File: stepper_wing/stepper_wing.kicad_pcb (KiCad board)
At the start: 2 copper layers, 47 x 49.5 mm, 39 parts, among them M1 Nylon, M2 Nylon, P1 24V, P2 GND, U1 MCP44X1, U2 MCP23017, U3 DRV8825, U4 DRV8825, U5 DRV8825, U6 DRV8825

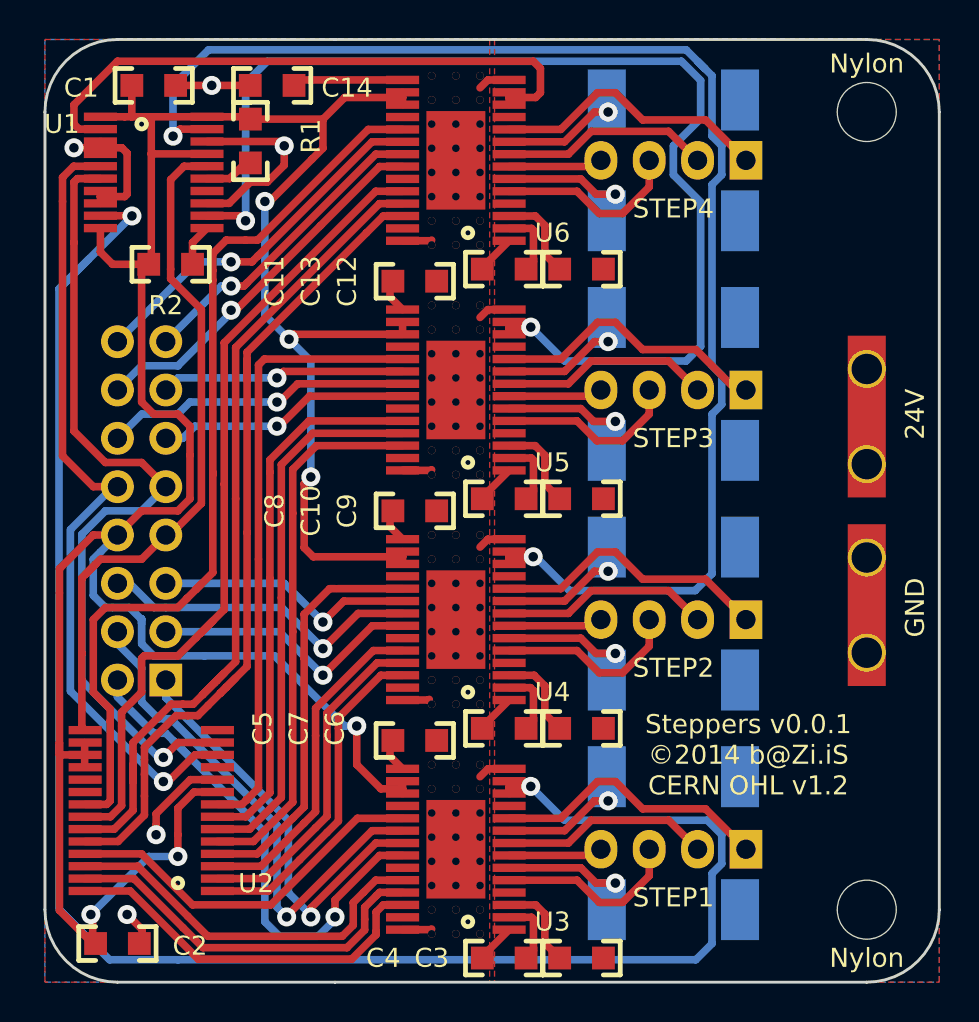
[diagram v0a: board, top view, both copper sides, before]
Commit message: more titdy
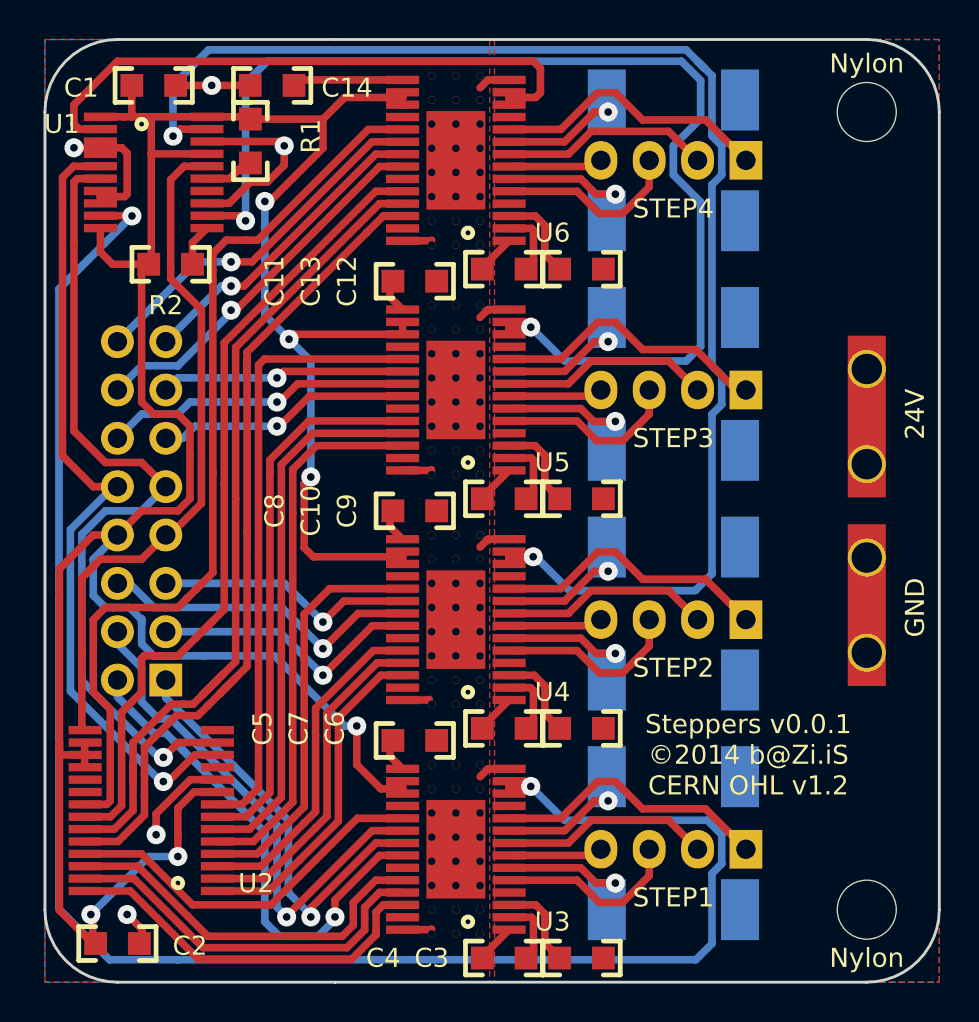
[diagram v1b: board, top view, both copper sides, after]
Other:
- net class Default: via_drill 0.5 -> 0.4
